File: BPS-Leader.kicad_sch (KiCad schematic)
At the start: 18 parts, among them J10 Fan2, J11 Fan3, J12 Fan4, J13 HV+ Connector, J14 HV- Connector, J15 Array Connector, J17 Fan5, J18 Strobe_Conn, J19 ADC SPI, J20 Fan I2C, J21 Segment1 Connector, J22 Segment2 Connector, J23 lSOMconn, J4 Fan I2C, J8 E-STOP, J9 Fan1, U1 PeripheralSOM

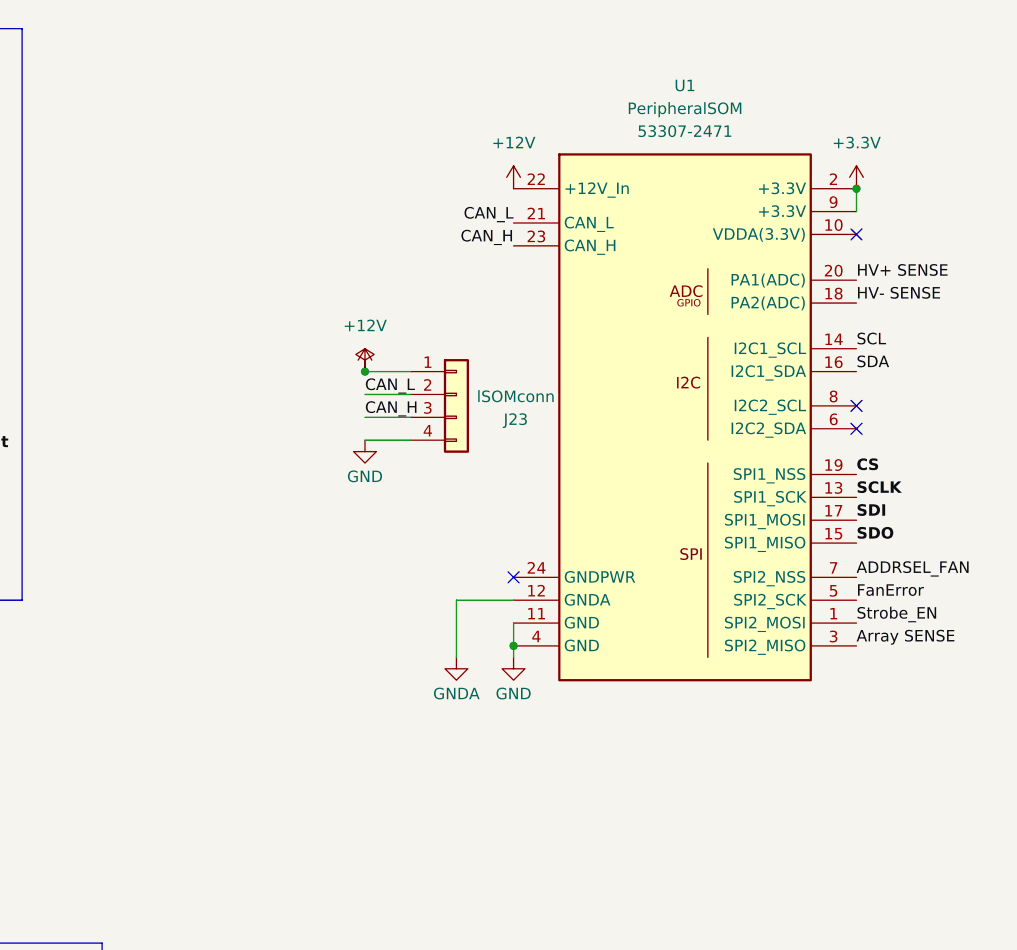
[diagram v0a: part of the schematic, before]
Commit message: need to find a spot for the 3 new connectors and also flip the old connectors and also finish traces to leadersom
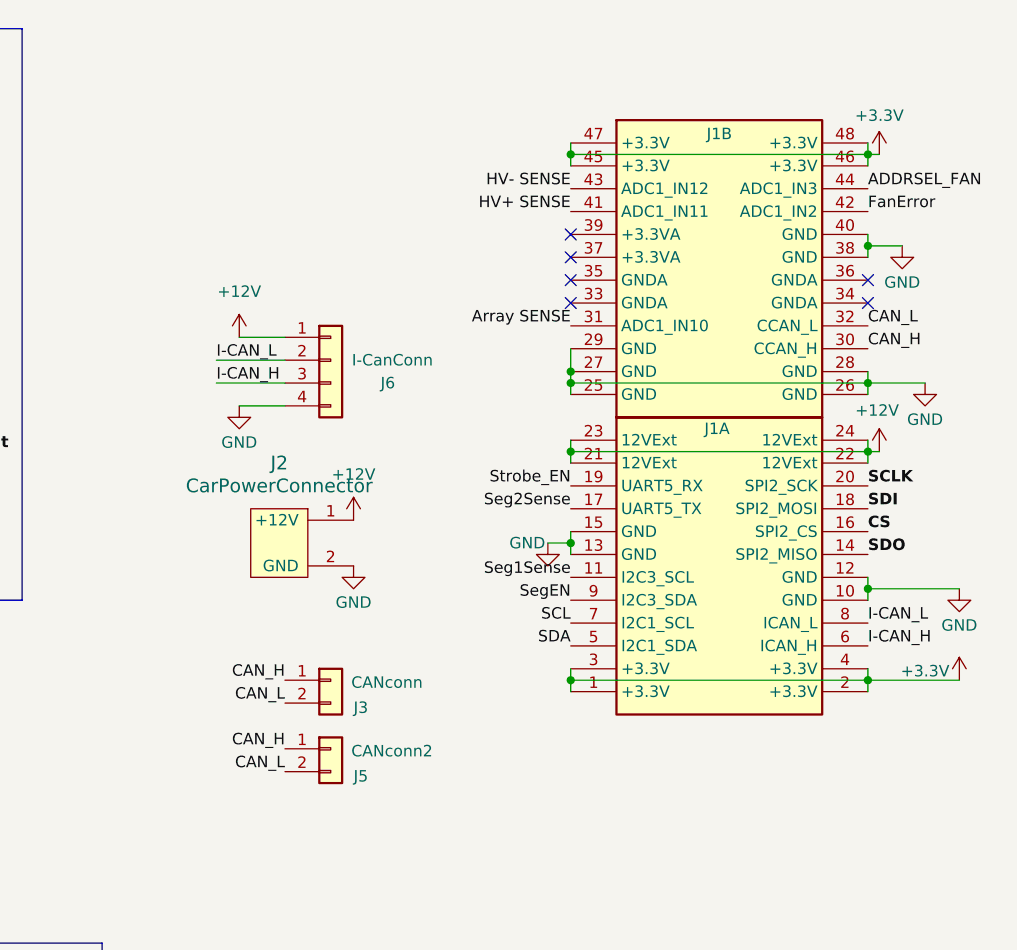
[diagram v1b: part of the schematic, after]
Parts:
- removed J23: lSOMconn, Connector_Molex:Molex_Micro-Fit_3.0_43650-0415_1x04_P3.00mm_Vertical, symbol Connector_Generic:Conn_01x04
- removed U1: PeripheralSOM, UTSVT_Special:PeripheralSOM, symbol utsvt-misc:PeripheralSOM
- added J1: ~, UTSVT_Special:LeaderSOM, symbol utsvt-connectors:LSOM_DaughterConn
- added J2: CarPowerConnector, Connector_Molex:Molex_Micro-Fit_3.0_43650-0215_1x02_P3.00mm_Vertical, symbol utsvt-connectors:CarPowerConnector
- added J3: CANconn, Connector_Molex:Molex_Micro-Fit_3.0_43650-0215_1x02_P3.00mm_Vertical, symbol Connector_Generic:Conn_01x02
- added J5: CANconn2, Connector_Molex:Molex_Micro-Fit_3.0_43650-0215_1x02_P3.00mm_Vertical, symbol Connector_Generic:Conn_01x02
- added J6: I-CanConn, Connector_Molex:Molex_Micro-Fit_3.0_43650-0415_1x04_P3.00mm_Vertical, symbol Connector_Generic:Conn_01x04
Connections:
- net +12V: now also J1.21 (12VExt), J1.22 (12VExt), J1.23 (12VExt), J1.24 (12VExt), J2.1 (+12V), J6.1 (Pin_1)
- net +3.3V: now also J1.1 (+3.3V), J1.2 (+3.3V), J1.3 (+3.3V), J1.4 (+3.3V), J1.45 (+3.3V), J1.46 (+3.3V), J1.47 (+3.3V), J1.48 (+3.3V)
- net ADDRSEL_FAN: now also J1.44 (ADC1_IN3)
- net Array SENSE: now also J1.31 (ADC1_IN10)
- net CAN_H: now also J1.30 (CCAN_H), J3.1 (Pin_1), J5.1 (Pin_1)
- net CAN_L: now also J1.32 (CCAN_L), J3.2 (Pin_2), J5.2 (Pin_2)
- net CS: now also J1.16 (SPI2_CS)
- net FanError: now also J1.42 (ADC1_IN2)
- net GND: now also J1.10 (GND), J1.12 (GND), J1.13 (GND), J1.15 (GND), J1.25 (GND), J1.26 (GND), J1.27 (GND), J1.28 (GND), J1.29 (GND), J1.38 (GND), J1.40 (GND), J2.2 (GND), J6.4 (Pin_4)
- net HV+ SENSE: now also J1.41 (ADC1_IN11)
- net HV- SENSE: now also J1.43 (ADC1_IN12)
- net SCL: now also J1.7 (I2C1_SCL)
- net SCLK: now also J1.20 (SPI2_SCK)
- net SDA: now also J1.5 (I2C1_SDA)
- net SDI: now also J1.18 (SPI2_MOSI)
- net SDO: now also J1.14 (SPI2_MISO)
- net Seg1Sense: now also J1.11 (I2C3_SCL)
- net Seg2Sense: now also J1.17 (UART5_TX)
- net SegEN: now also J1.9 (I2C3_SDA)
- net Strobe_EN: now also J1.19 (UART5_RX)
- new net I-CAN_H: J1.6 (ICAN_H), J6.3 (Pin_3)
- new net I-CAN_L: J1.8 (ICAN_L), J6.2 (Pin_2)
- no-connect marks 4 -> 6
